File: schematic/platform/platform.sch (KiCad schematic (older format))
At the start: 4 parts, among them J1 PLATFORM_CONNECTOR, J2 KY-018 PHOTORESISTOR MODULE, U1 HC-SR04

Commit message: Migrate to STM32F411 + add HC-SR04
+ Add support of HC-SR04 ultrasound sensor
+ Update the virtual registers library
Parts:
- removed A1: Arduino_Nano_v3.x, Module:Arduino_Nano, symbol MCU_Module:Arduino_Nano_v3.x
- removed J1: PLATFORM_CONNECTOR, symbol Connector:Conn_01x08_Female
- removed J2: KY-018 PHOTORESISTOR MODULE, symbol Connector:Conn_01x03_Male
- removed U1: HC-SR04, XCVR_HC-SR04, symbol HC-SR04:HC-SR04
- added BT1: PowerBank_1xOUT, symbol zk_modules:PowerBank_1xOUT
- added J1: Conn_ZKP_1.3, symbol zk_connectors:Conn_ZKP_1.3
- added U1: STM32F411RETx, Package_QFP:LQFP-64_10x10mm_P0.5mm, symbol MCU_ST_STM32F4:STM32F411RETx
- added U2: HC-SR04, XCVR_HC-SR04, symbol zk_modules:HC-SR04
- added U3: KY-018, symbol zk_modules:KY-018
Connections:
- net labels added: PHOTO_SIGNAL
- wire segments 21 -> 17
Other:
- note removed: "+3V OUT"
- note removed: "+5V IN"
- note removed: "+5V OUT"
- note removed: "GND"
- note removed: "RESET"
- note removed: "SCK"
- note removed: "SDA"
- note removed: "SIGNAL"
- note removed: "VCC"

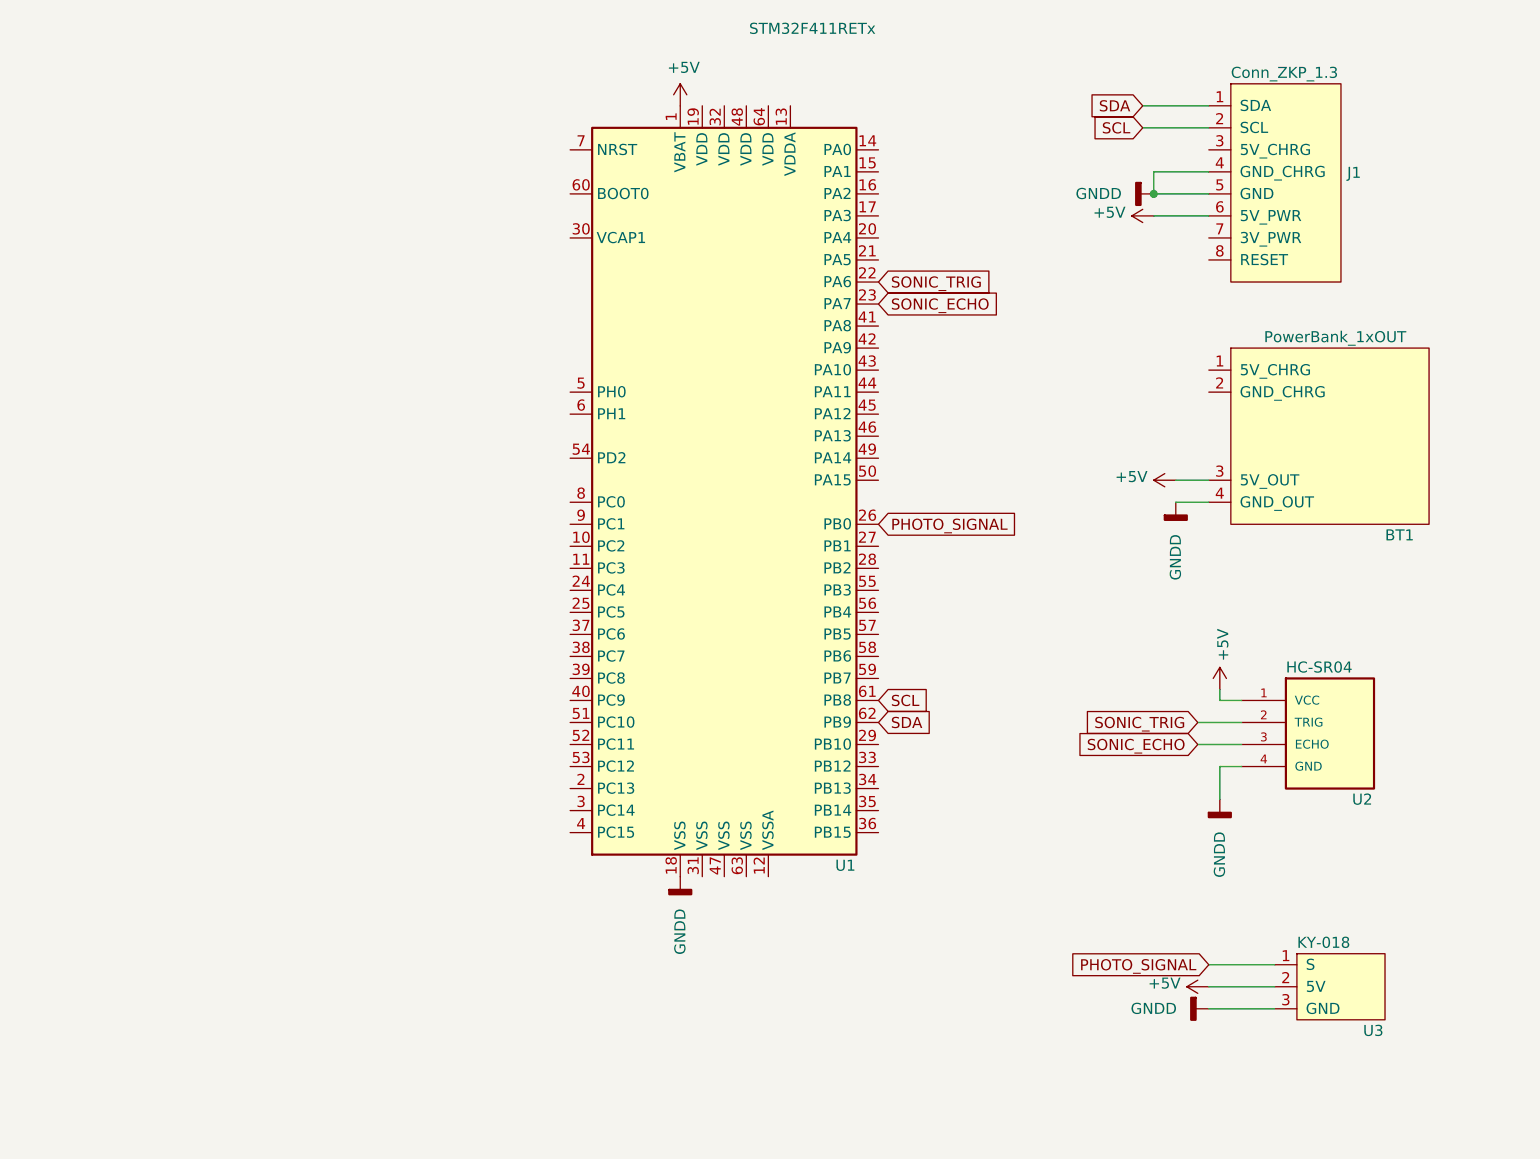
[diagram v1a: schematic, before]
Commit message: Update schematic
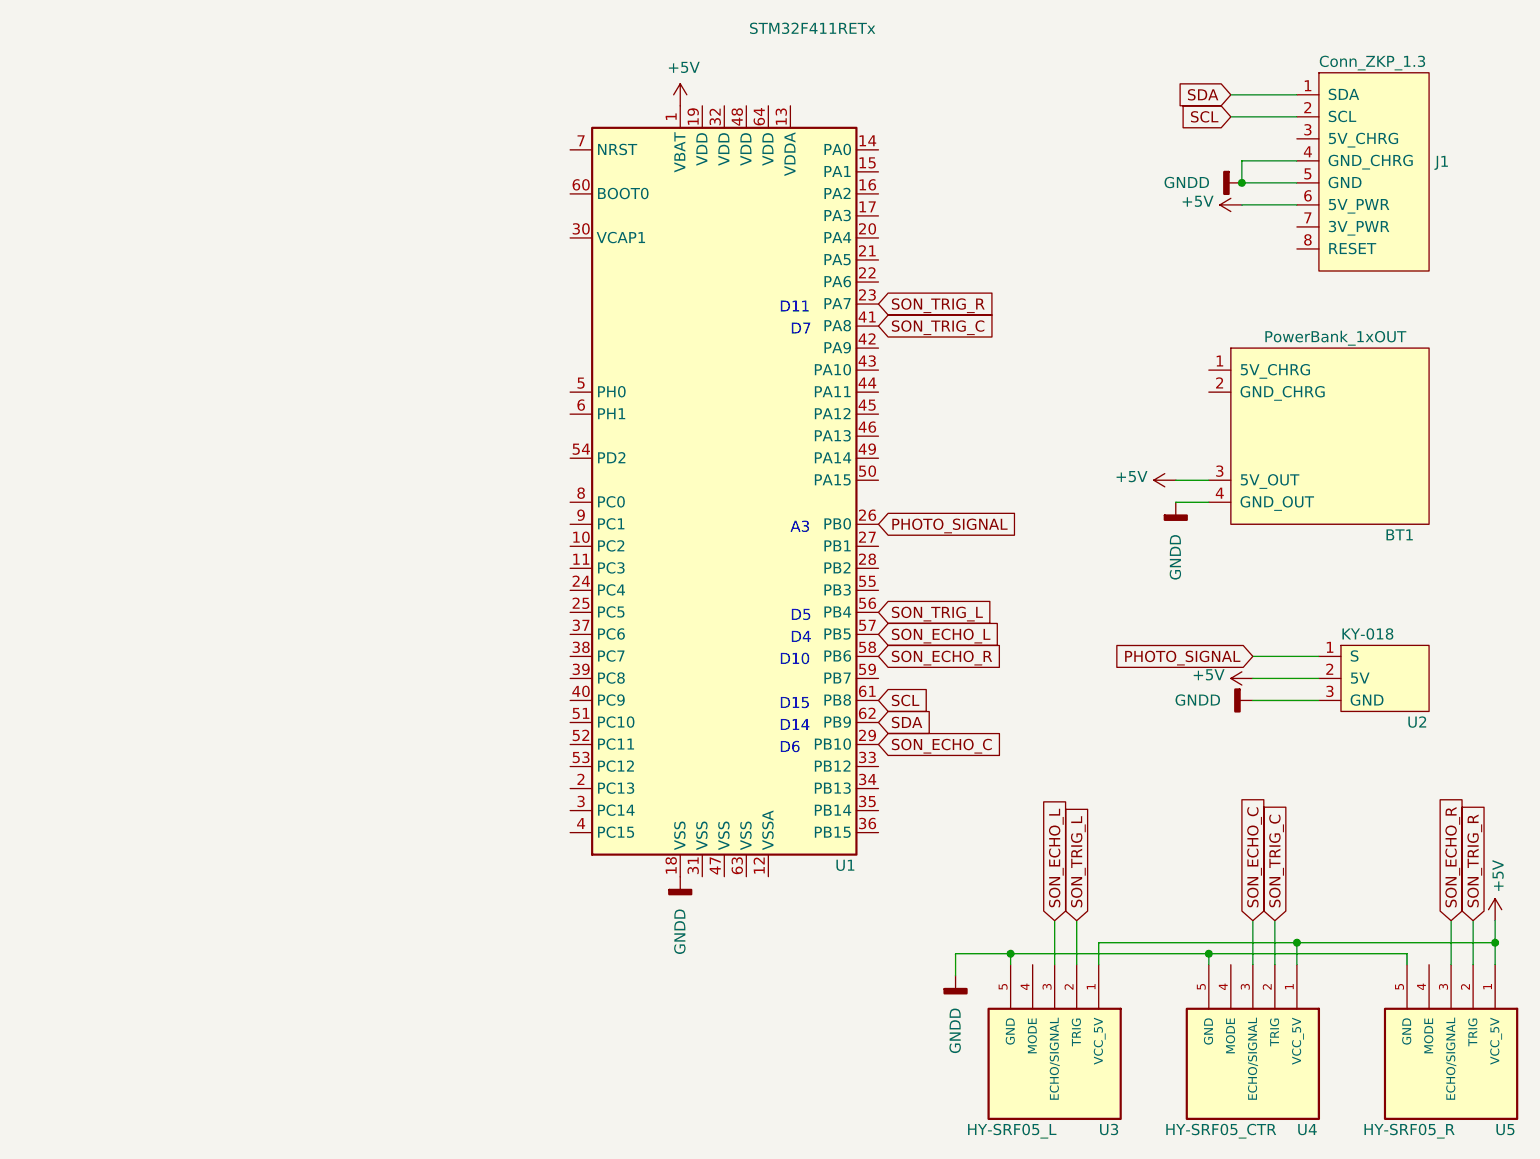
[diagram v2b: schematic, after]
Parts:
- removed U2: HC-SR04, XCVR_HC-SR04, symbol zk_modules:HC-SR04
- added U3: HY-SRF05_L, XCVR_HC-SR04, symbol zk_modules:HY-SRF05
- added U4: HY-SRF05_CTR, XCVR_HC-SR04, symbol zk_modules:HY-SRF05
- added U5: HY-SRF05_R, XCVR_HC-SR04, symbol zk_modules:HY-SRF05
- renumbered U3 to U2
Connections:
- net +5V: now also U3.1 (VCC_5V), U4.1 (VCC_5V), U5.1 (VCC_5V)
- net GNDD: now also U3.5 (GND), U4.5 (GND), U5.5 (GND)
- net SON_ECHO_C: now reaches U1.29 (PB10)
- net SON_ECHO_C: now also U4.3 (ECHO/SIGNAL)
- net SON_TRIG_C: now reaches U1.41 (PA8)
- net SON_TRIG_C: now also U4.2 (TRIG)
- net SON_TRIG_L: now reaches U1.56 (PB4)
- net SON_TRIG_L: now also U3.2 (TRIG)
- net SON_ECHO_L: now reaches U1.57 (PB5)
- net SON_ECHO_L: now also U3.3 (ECHO/SIGNAL)
- net SON_ECHO_R: now reaches U1.58 (PB6)
- net SON_ECHO_R: now also U5.3 (ECHO/SIGNAL)
- net SONIC_ECHO renamed SON_TRIG_R
- net SON_TRIG_R: now also U5.2 (TRIG)
- net SONIC_TRIG: no longer names the net of U1.22 (PA6)
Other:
- note added: "A3"
- note added: "D10"
- note added: "D11"
- note added: "D14"
- note added: "D15"
- note added: "D4"
- note added: "D5"
- note added: "D6"
- note added: "D7"
- moved on the sheet: J1, U2
